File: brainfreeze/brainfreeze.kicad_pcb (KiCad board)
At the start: 4 copper layers, 69.6 x 106.9 mm, 13 parts, among them J1 XT30PW-M, P1 OSTTE020104, Q1 DMN63D8L-7, U1 H3LIS331DL, U3 AP63205WU

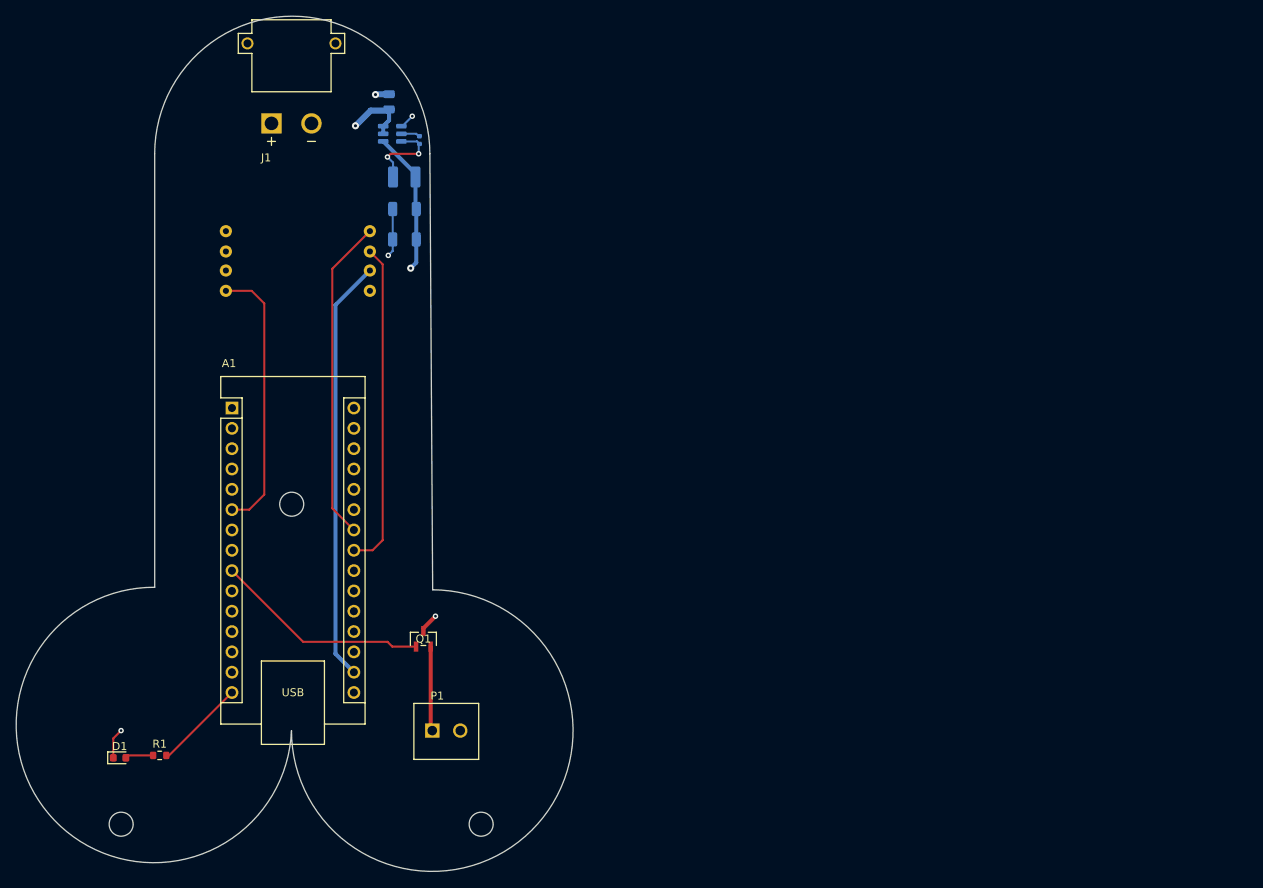
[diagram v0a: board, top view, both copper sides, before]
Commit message: Created gerber files
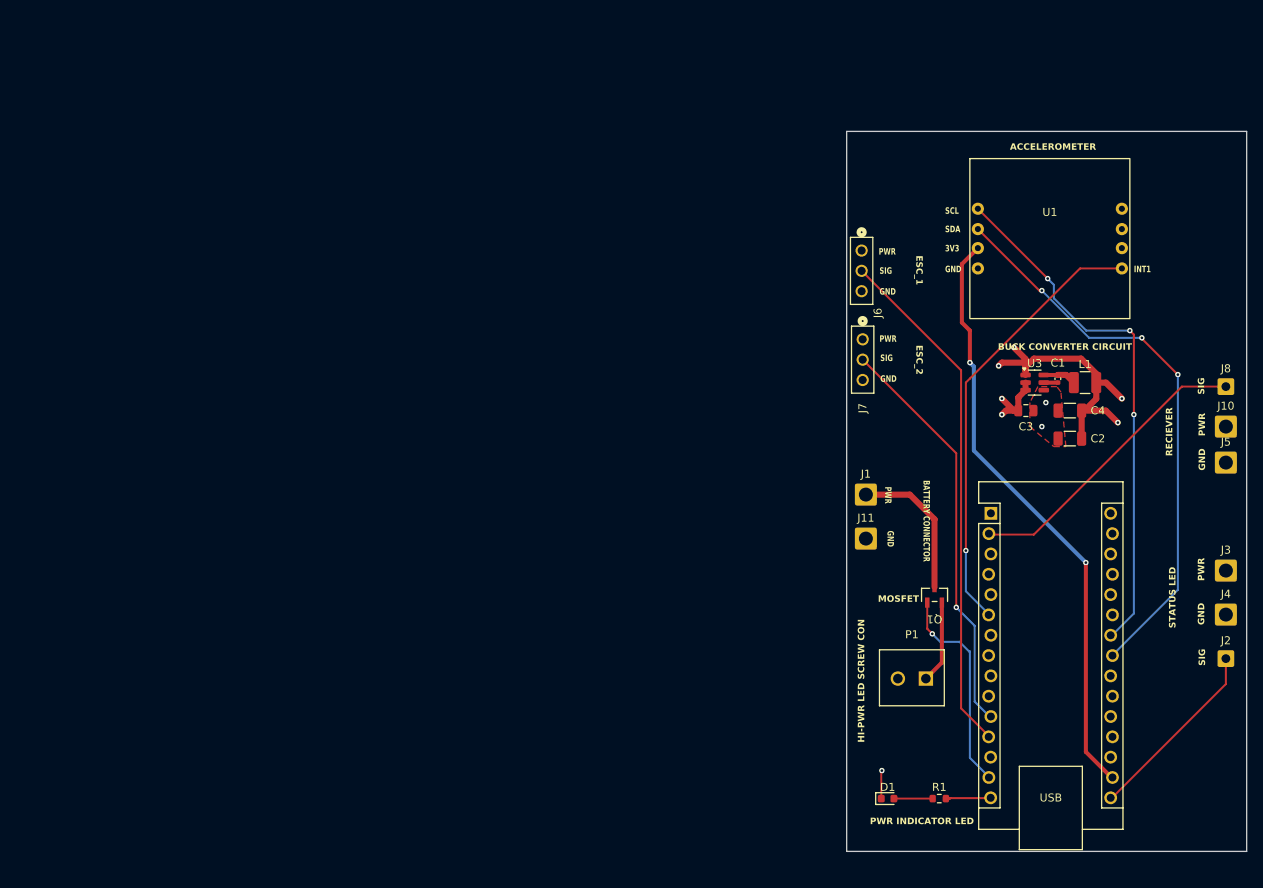
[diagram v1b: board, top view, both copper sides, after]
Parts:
- added G***: LOGO, brainfreeze:frost.image, B.Cu at (200.6, 110.4)
- added J10: Conn_01x01_Pin, Connector_Wire:SolderWire-1sqmm_1x01_D1.4mm_OD2.7mm, F.Cu at (222.5, 103.5)
- added J11: Conn_01x01_Pin, Connector_Wire:SolderWire-1sqmm_1x01_D1.4mm_OD2.7mm, F.Cu at (177.5, 117.5)
- added J2: Conn_01x01_Pin, Connector_Wire:SolderWire-0.5sqmm_1x01_D0.9mm_OD2.1mm, F.Cu at (222.5, 132.5)
- added J3: Conn_01x01_Pin, Connector_Wire:SolderWire-1sqmm_1x01_D1.4mm_OD2.7mm, F.Cu at (222.5, 121.5)
- added J4: Conn_01x01_Pin, Connector_Wire:SolderWire-1sqmm_1x01_D1.4mm_OD2.7mm, F.Cu at (222.5, 127.0)
- added J5: Conn_01x01_Pin, Connector_Wire:SolderWire-1sqmm_1x01_D1.4mm_OD2.7mm, F.Cu at (222.5, 108.0)
- added J6: Conn_01x03_Socket, brainfreeze:ESC CON, F.Cu at (177.0, 81.5)
- added J7: Conn_01x03_Socket, brainfreeze:ESC CON, F.Cu at (177.1, 92.6)
- added J8: Conn_01x01_Pin, Connector_Wire:SolderWire-0.5sqmm_1x01_D0.9mm_OD2.1mm, F.Cu at (222.5, 98.5)
- A1: footprint Module:Arduino_Nano -> brainfreeze:NANO_FIT
- C1, C2, C3, C4, L1, U1, U3: moved to F.Cu
- J1: value XT30PW-M -> Conn_01x01_Pin; footprint brainfreeze:XT30PW-M -> Connector_Wire:SolderWire-1sqmm_1x01_D1.4mm_OD2.7mm
- moved A1 110.9 mm to (201.3, 142.0)
- moved R1 97.6 mm to (186.7, 150.0)
- moved D1 96.1 mm to (180.2, 150.0)
- moved U1 94.0 mm to (200.5, 80.0), turned to 0 degrees
- moved J1 91.3 mm to (177.5, 112.0)
- moved L1 88.9 mm to (204.9, 98.0)
- moved C3 88.5 mm to (197.5, 101.5), turned to 0 degrees
- moved C2 88.0 mm to (203.0, 105.0)
- moved U3 86.1 mm to (198.6, 98.0)
- moved C4 85.9 mm to (203.0, 101.5)
- moved C1 85.2 mm to (201.5, 97.5), turned to -90 degrees
- moved Q1 64.1 mm to (186.1, 124.5)
- moved P1 58.6 mm to (183.2, 135.0), turned to 180 degrees
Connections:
- A1 pad 11: unconnected-(A1-D8-Pad11) -> ESC_2
- A1 pad 12: unconnected-(A1-D9-Pad12) -> ESC_1
- A1 pad 14: unconnected-(A1-D11-Pad14) -> LED
- A1 pad 16: unconnected-(A1-D13-Pad16) -> NEOPIXEL LED
- A1 pad 2: unconnected-(A1-D0/RX-Pad2) -> RX
- A1 pad 21: unconnected-(A1-A2-Pad21) -> ESC_SIGNAL2
- A1 pad 22: unconnected-(A1-A3-Pad22) -> ESC_SIGNAL3
- A1 pad 5: unconnected-(A1-D2-Pad5) -> ESC_SIGNAL1
- A1 pad 9: LED -> unconnected-(A1-D6-Pad9)
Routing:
- net ESC_1: track 0.00 -> 64.9 mm
- net ESC_2: track 0.00 -> 51.2 mm, vias 0 -> 1
- net RX: track 0.00 -> 37.2 mm
- net SDA: track 40.9 -> 71.2 mm, vias 0 -> 3
- net SCL: track 40.4 -> 65.8 mm, vias 0 -> 3
- net NEOPIXEL LED: track 0.00 -> 23.6 mm
- net 3V3: track 52.9 -> 74.8 mm, vias 0 -> 2
- net INT1: track 34.2 -> 55.7 mm, vias 0 -> 1
- net +5V: track 17.9 -> 36.0 mm, vias 1 -> 4
- net +12V: track 10.9 -> 27.2 mm
- net GND: track 13.4 -> 3.53 mm, vias 4 -> 3
- net Net-(U3-BST): track 10.5 -> 4.16 mm, vias 2 -> 0
- net Net-(A1-D12): track 11.7 -> 5.52 mm
- net Net-(D1-A): track 3.74 -> 4.85 mm
- net Net-(U3-SW): track 2.29 -> 1.76 mm
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- added copper zone on F.Cu, net GND
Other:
- board size 69.6 x 106.9 mm -> 50 x 90 mm
- board text added: "3V3"
- board text added: "ACCELEROMETER"
- board text added: "BATTERY CONNECTOR"
- board text added: "BUCK CONVERTER CIRCUIT"
- board text added: "DESIGNED BY: Nathaniel Wheeler, Kamran Isfahani AND Pedro Coelho FOR UCONN FROST ROBOTICS"
- board text added: "ESC_1"
- board text added: "ESC_2"
- board text added: "GND"
- board text added: "HI-PWR LED SCREW CON"
- board text added: "INT1"
- board text added: "MOSFET"
- board text added: "PWR"
- board text added: "PWR INDICATOR LED"
- board text added: "RECIEVER"
- board text added: "SCL"
- board text added: "SDA"
- board text added: "SIG"
- board text added: "STATUS LED"
